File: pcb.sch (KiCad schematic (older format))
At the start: 76 parts, among them SW1 SW_Push, U1 ATmega32U4-AU, Y1 16MHz

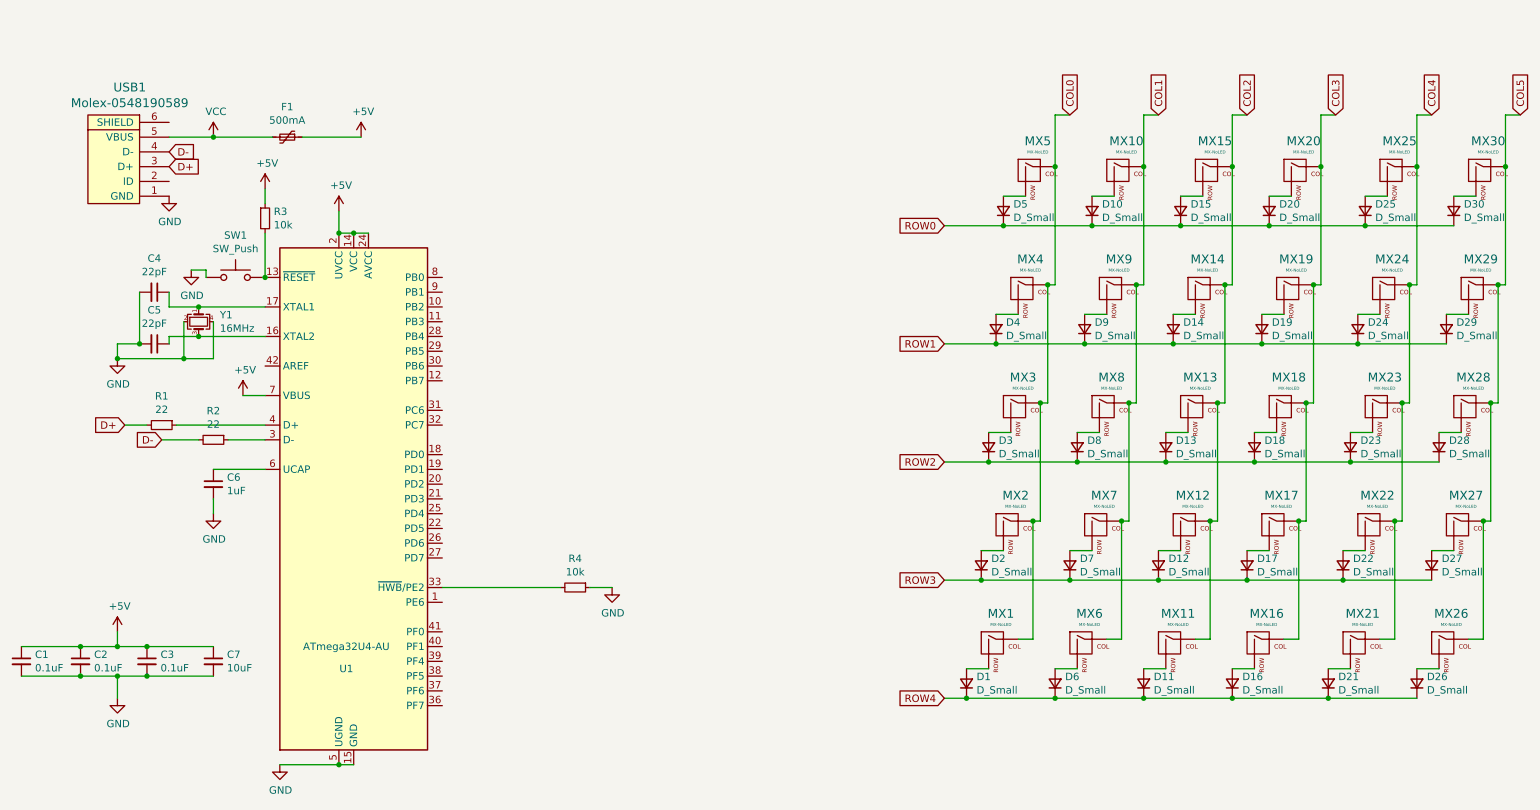
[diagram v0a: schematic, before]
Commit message: No idea
No clue what's changed
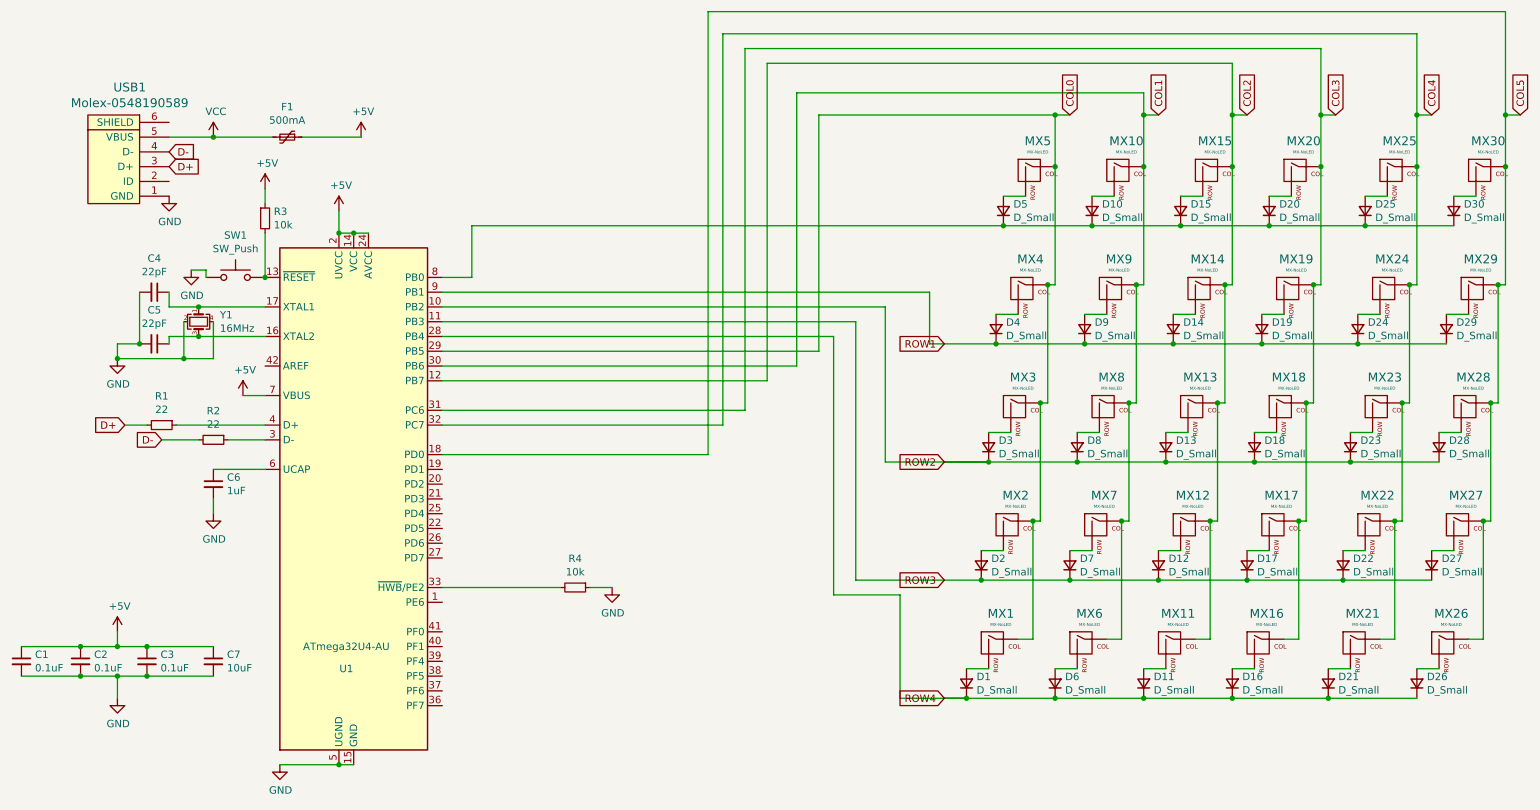
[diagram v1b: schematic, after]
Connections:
- net ROW0 is gone; now on an unnamed net: D10.1 (K), D15.1 (K), D20.1 (K), D25.1 (K), D30.1 (K), D5.1 (K)
- net COL0: now also U1.29 (PB5)
- net COL1: now also U1.30 (PB6)
- net COL2: now also U1.12 (PB7)
- net COL3: now also U1.31 (PC6)
- net COL4: now also U1.32 (PC7)
- net COL5: now also U1.18 (PD0)
- net ROW1: now also U1.9 (PB1)
- net ROW2: now also U1.10 (PB2)
- net ROW3: now also U1.11 (PB3)
- net ROW4: now also U1.28 (PB4)
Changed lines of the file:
@@
 	7300 5050 7150 5050
-Wire Wire Line
-	7850 1300 7750 1300
 Wire Wire Line
 	7750 1300 7750 1650
@@
 Connection ~ 10650 4050
 Wire Wire Line
-	7000 2050 7400 2050
-Wire Wire Line
 	7400 2050 8000 2050
-Connection ~ 7400 2050
 Wire Wire Line
 	8000 2050 8600 2050
@@
 Connection ~ 9850 2050
 Wire Wire Line
-	7000 2850 7350 2850
-Wire Wire Line
 	7350 2850 7950 2850
 Connection ~ 7350 2850
@@
 Connection ~ 9800 2850
 Wire Wire Line
-	7000 3650 7300 3650
-Wire Wire Line
 	7300 3650 7900 3650
 Connection ~ 7300 3650
@@
 Connection ~ 9750 3650
 Wire Wire Line
-	7000 4450 7250 4450
-Wire Wire Line
 	7250 4450 7850 4450
 Connection ~ 7250 4450
@@
 	9700 4450 10300 4450
 Connection ~ 9700 4450
-Wire Wire Line
-	7000 5250 7150 5250
 Connection ~ 7150 5250
 Wire Wire Line
@@
 Text GLabel 10900 1300 1    50   Input ~ 0
 COL5
-Text GLabel 7000 2050 0    50   Input ~ 0
-ROW0
 Text GLabel 7000 2850 0    50   Input ~ 0
 ROW1
@@
 	1    0    0    -1
 $EndComp
+Wire Wire Line
+	3800 2400 3600 2400
+Wire Wire Line
+	7400 2050 3800 2050
+Wire Wire Line
+	3800 2050 3800 2400
+Connection ~ 7400 2050
+Wire Wire Line
+	6900 2850 6900 2500
+Wire Wire Line
+	6900 2500 3600 2500
+Wire Wire Line
+	3600 2600 6600 2600
+Wire Wire Line
+	6600 2600 6600 3650
+Wire Wire Line
+	6900 2850 7350 2850
+Wire Wire Line
+	6400 4450 6400 2700
+Wire Wire Line
+	6400 2700 3600 2700
+Wire Wire Line
+	3600 2800 6250 2800
+Wire Wire Line
+	6250 2800 6250 4550
+Wire Wire Line
+	6250 4550 6700 4550
+Wire Wire Line
+	6700 4550 6700 5250
+Wire Wire Line
+	7000 3650 7300 3650
+Wire Wire Line
+	6400 4450 7250 4450
+Wire Wire Line
+	6600 3650 7300 3650
+Wire Wire Line
+	7000 5250 7150 5250
+Wire Wire Line
+	7850 1300 7750 1300
+Wire Wire Line
+	7750 1300 6150 1300
+Wire Wire Line
+	6150 1300 6150 2900
+Wire Wire Line
+	6150 2900 3600 2900
+Wire Wire Line
+	6700 5250 7150 5250
+Connection ~ 7750 1300
+Wire Wire Line
+	8350 1300 8350 1150
+Wire Wire Line
+	8350 1150 6000 1150
+Wire Wire Line
+	6000 1150 6000 3000
+Wire Wire Line
+	6000 3000 3600 3000
+Connection ~ 8350 1300
+Wire Wire Line
+	8950 1300 8950 950
+Wire Wire Line
+	8950 950  5800 950
+Wire Wire Line
+	5800 950  5800 3100
+Wire Wire Line
+	5800 3100 3600 3100
+Connection ~ 8950 1300
+Wire Wire Line
+	9550 1300 9550 850
+Wire Wire Line
+	9550 850  5650 850
+Wire Wire Line
+	5650 850  5650 3300
+Wire Wire Line
+	5650 3300 3600 3300
+Connection ~ 9550 1300
+Wire Wire Line
+	3600 3400 5500 3400
+Wire Wire Line
+	5500 3400 5500 750
+Wire Wire Line
+	5500 750  10200 750
+Wire Wire Line
+	10200 750  10200 1300
+Connection ~ 10200 1300
+Wire Wire Line
+	10800 1300 10800 600
+Wire Wire Line
+	10800 600  5400 600
+Wire Wire Line
+	5400 600  5400 3600
+Wire Wire Line
+	5400 3600 3600 3600
+Connection ~ 10800 1300
 $EndSCHEMATC
